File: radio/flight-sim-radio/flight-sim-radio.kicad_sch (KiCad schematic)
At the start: 30 parts, among them J1 Conn_01x03, J2 Conn_01x09, J3 Conn_01x04, SW1 RS-08 300±150GF, SW2 RotaryEncoder_Switch, SW3 RotaryEncoder_Switch, U1 74LS148, U3 TM1638, U4 TM1638

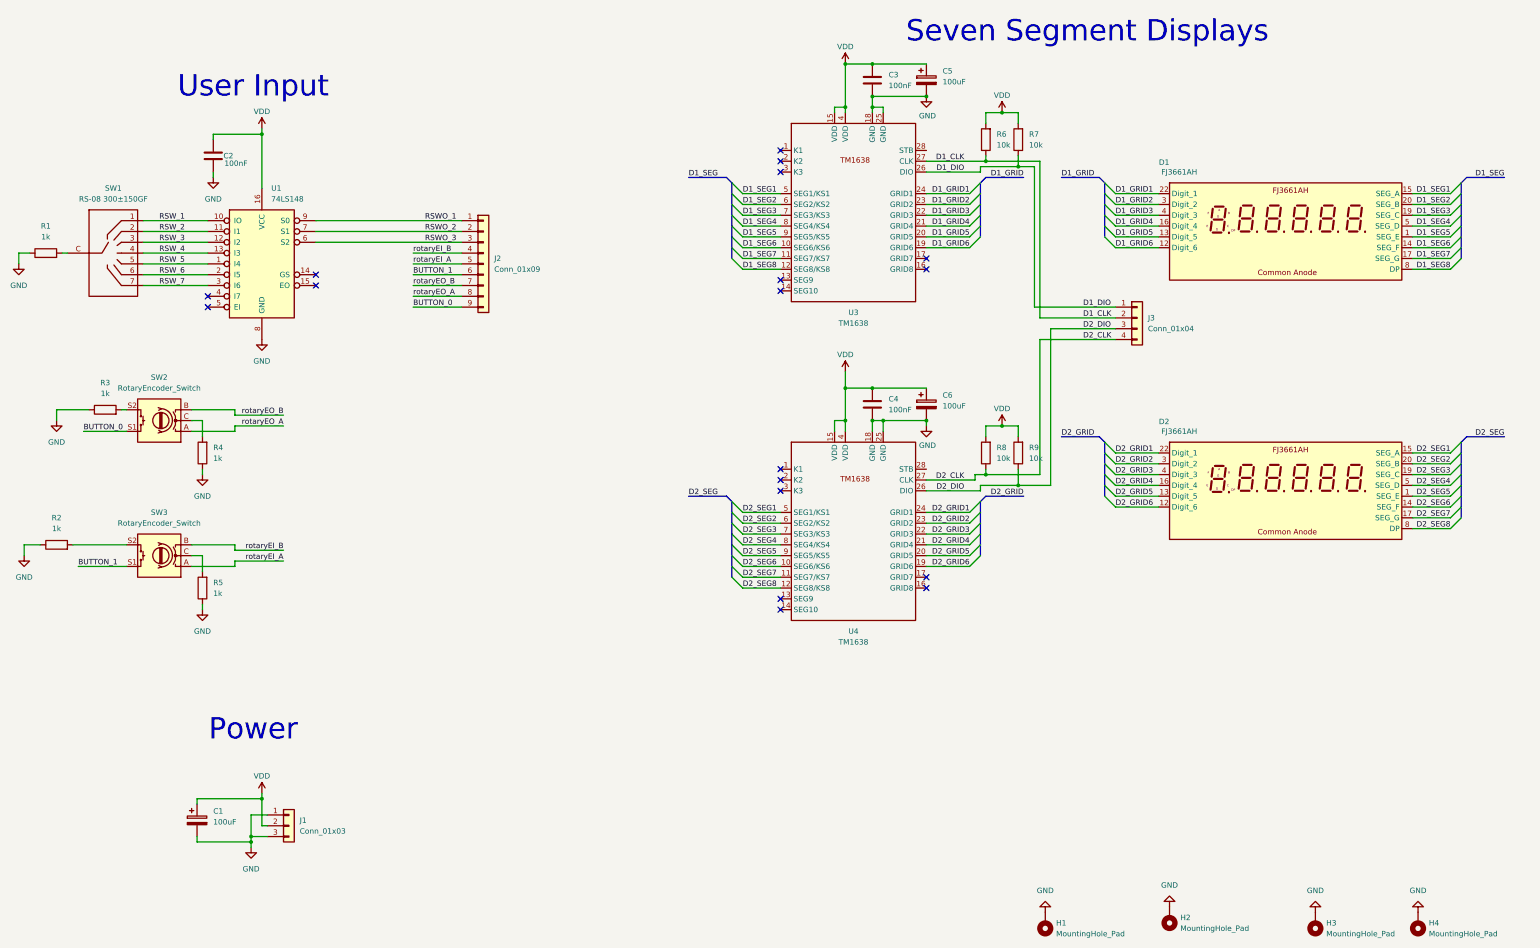
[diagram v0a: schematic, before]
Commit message: PCB complete
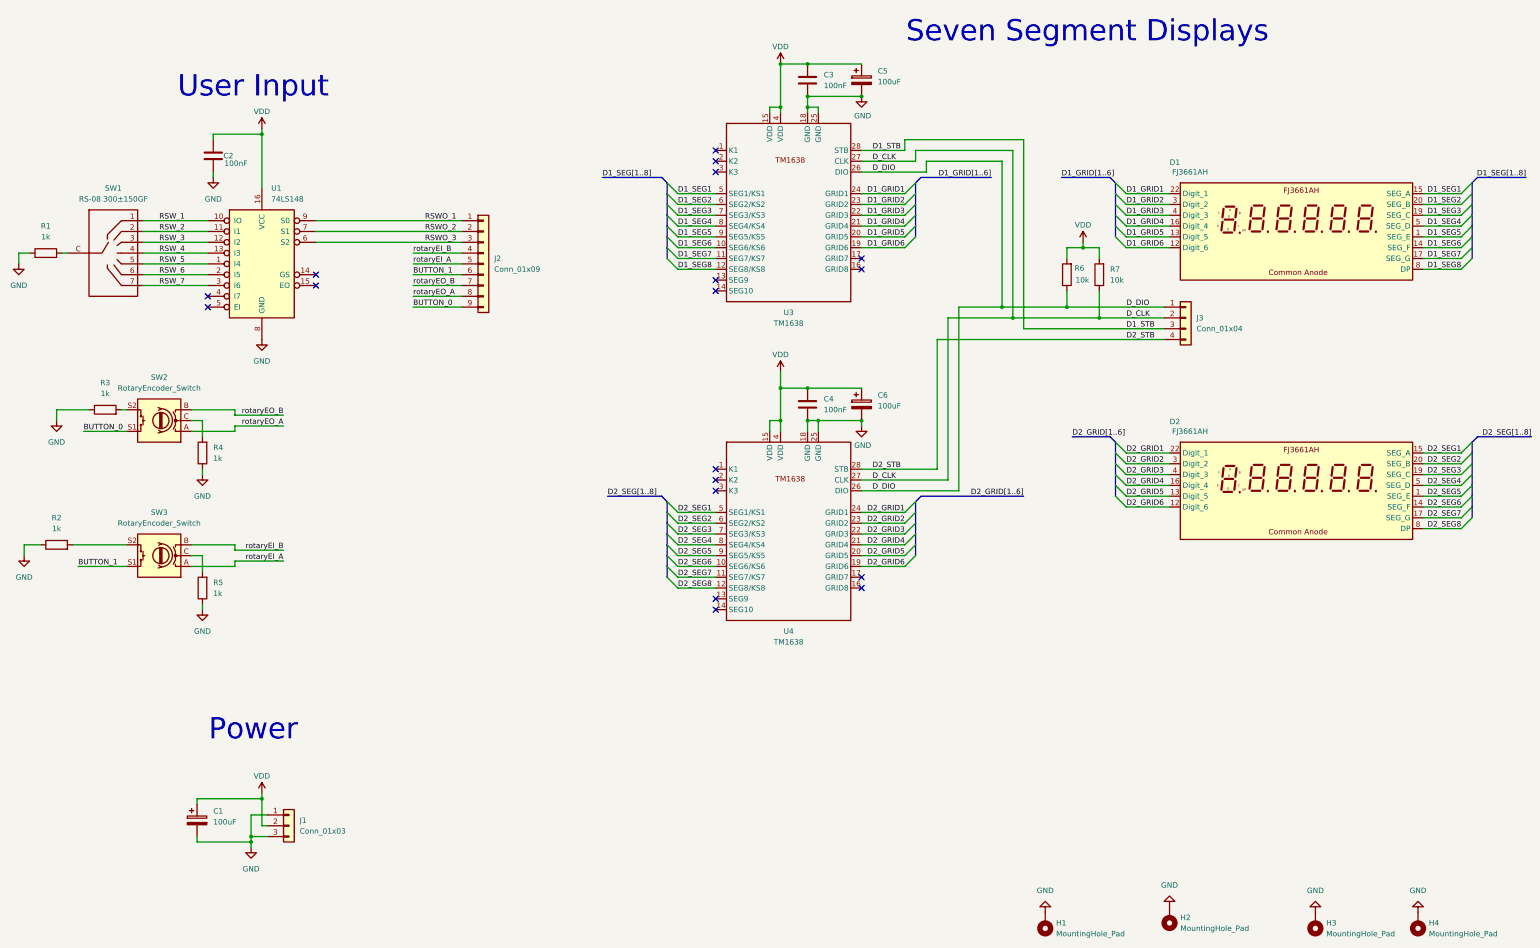
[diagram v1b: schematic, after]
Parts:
- removed R8, R9: 10k, Resistor_THT:R_Axial_DIN0207_L6.3mm_D2.5mm_P10.16mm_Horizontal, symbol Device:R
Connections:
- net D2_STB: now reaches U4.28 (STB)
- net D2_STB: now also J3.4 (Pin_4)
- net D1_STB: now reaches U3.28 (STB)
- net D1_STB: now also J3.3 (Pin_3)
- net D1_CLK renamed D_CLK
- net D_CLK: now also R7.1, U4.27 (CLK); no longer R6.1
- net D1_DIO renamed D_DIO
- net D_DIO: now also R6.1, U4.26 (DIO); no longer R7.1
- removed net D2_CLK: J3.4 (Pin_4), U4.27 (CLK)
- removed net D2_DIO: J3.3 (Pin_3), U4.26 (DIO)
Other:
- moved on the sheet: C3, C4, C5, C6, D1, D2, J3, U3, U4
